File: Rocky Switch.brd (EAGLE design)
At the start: 81.1 x 50.2 mm, 40 parts, among them T1 BTA16, T2 BTA16, T3 BTA16, T4 BTA16

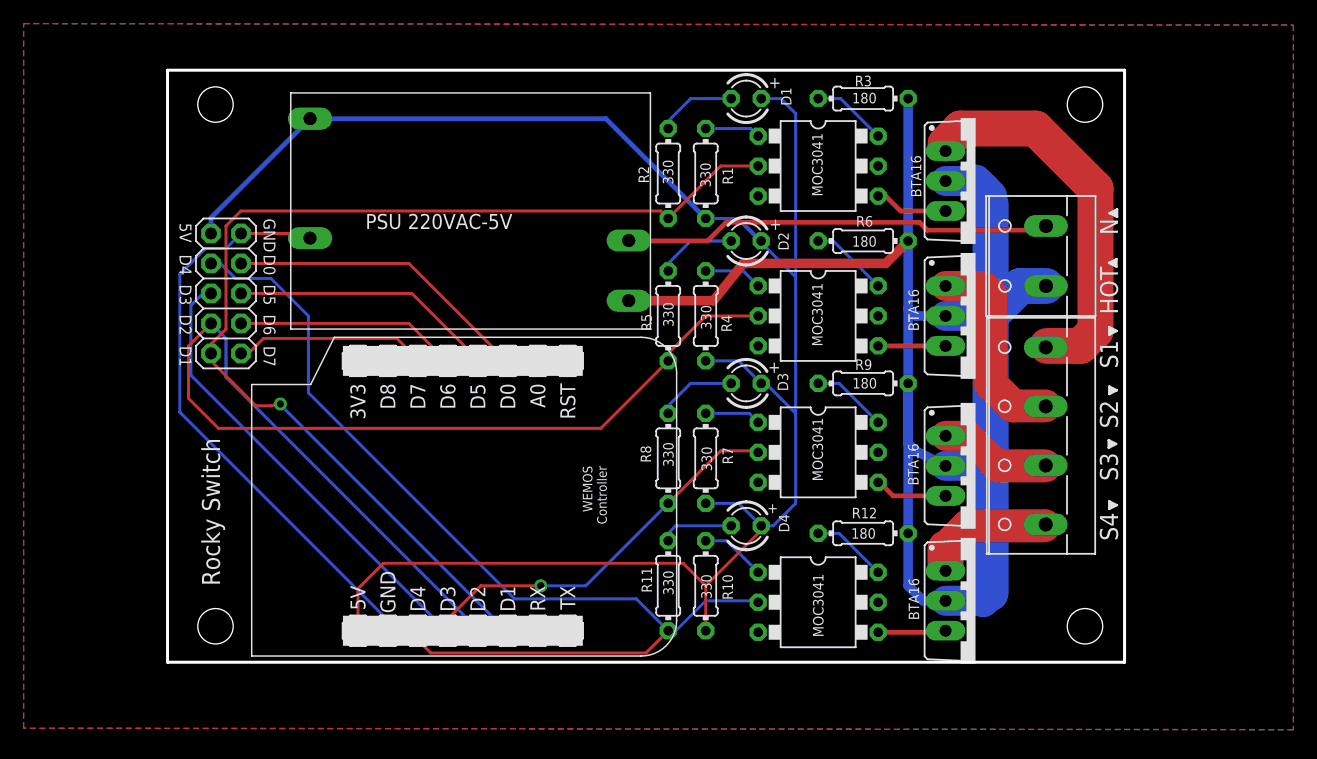
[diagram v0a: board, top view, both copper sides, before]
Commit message: Update board design to version 0.2
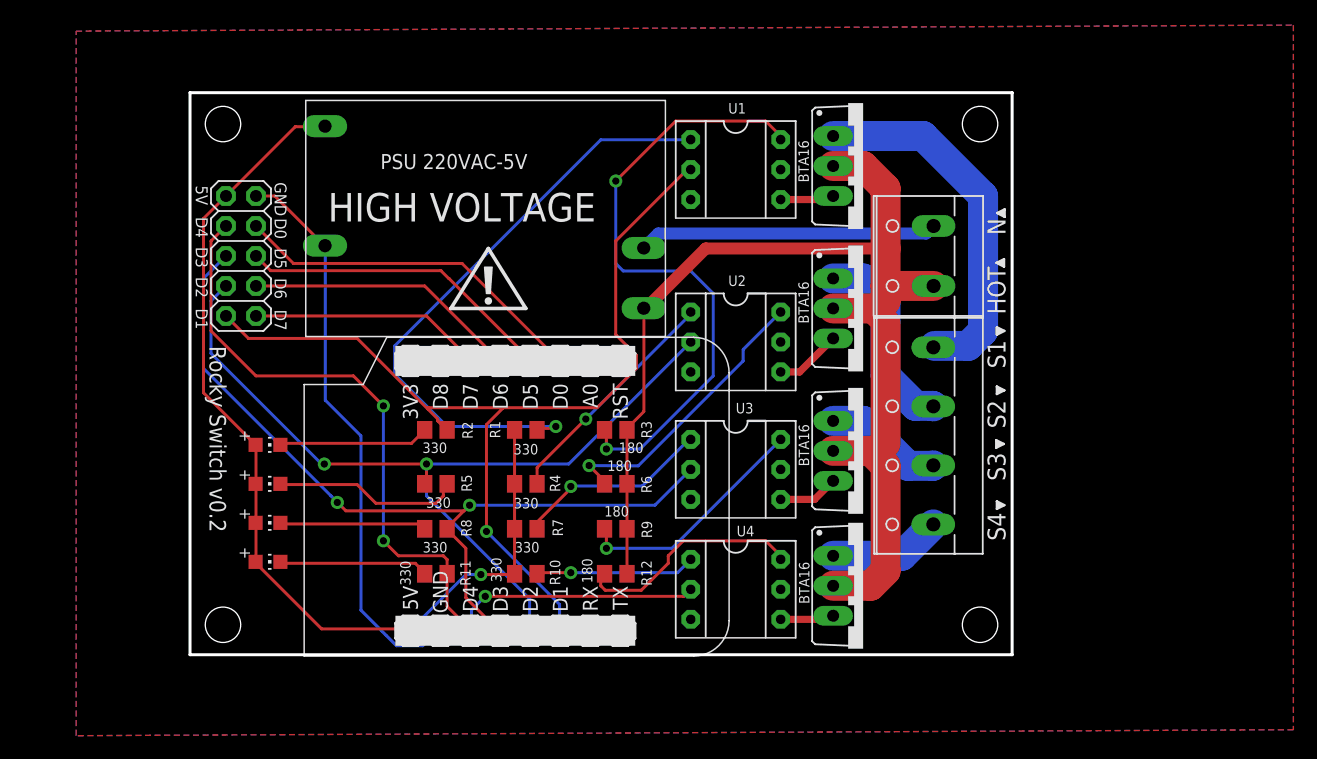
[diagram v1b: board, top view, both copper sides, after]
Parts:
- removed OK1, OK2, OK3, OK4: MOC3041, optocoupler:DIL06B
- added U1, U2, U3, U4: MOC3041, SparkFun-DiscreteSemi:DIL06
- D1: value (none) -> Relay1; device led:LED3MM -> adafruit:CHIP-LED0805
- D2: value (none) -> Relay2; device led:LED3MM -> adafruit:CHIP-LED0805
- D3: value (none) -> Relay3; device led:LED3MM -> adafruit:CHIP-LED0805
- D4: value (none) -> Relay4; device led:LED3MM -> adafruit:CHIP-LED0805
- R1, R10, R11, R12, R2, R3, R4, R5, R6, R7, R8, R9: device rcl:0204/7 -> rcl:R0805
- moved D1 50.0 mm to (9.27, 22.1), turned to 270 degrees
- moved D2 45.4 mm to (9.27, 18.8), turned to 270 degrees
- moved D3 42.2 mm to (9.27, 15.5), turned to 270 degrees
- moved D4 40.6 mm to (9.27, 12.2), turned to 270 degrees
- moved R3 35.0 mm to (38.7, 23.4)
- moved R6 29.4 mm to (38.7, 18.8)
- moved R2 29.3 mm to (23.5, 23.4), turned to 0 degrees
- moved R1 26.5 mm to (31.1, 23.4), turned to 0 degrees
- moved R9 24.3 mm to (38.7, 15.0)
- moved R5 24.3 mm to (23.5, 18.8), turned to 180 degrees
- moved U$17 21.3 mm to (27.9, 35.6), flipped to the top
- moved R12 21.2 mm to (38.7, 11.2)
- moved R4 20.8 mm to (31.1, 18.8), turned to 0 degrees
- moved R8 20.6 mm to (23.5, 15.0), turned to 0 degrees
- moved R11 19.7 mm to (23.5, 11.2), turned to 0 degrees
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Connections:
- net D1: now also U1.2; no longer OK1.2
- net D2: now also U2.2; no longer OK2.2
- net D3: now also U3.2; no longer OK3.2
- net D4: now also U4.2; no longer OK4.2
- net N$10: now also U1.1; no longer OK1.1
- net N$14: now also U1.6; no longer OK1.6
- net N$15: now also U2.4; no longer OK2.4
- net N$16: now also U2.1; no longer OK2.1
- net N$17: now also U2.6; no longer OK2.6
- net N$18: now also U3.4; no longer OK3.4
- net N$19: now also U3.1; no longer OK3.1
- net N$20: now also U3.6; no longer OK3.6
- net N$28: now also D1.C; no longer D1.K
- net N$29: now also D2.C; no longer D2.K
- net N$30: now also D3.C; no longer D3.K
- net N$32: now also U4.4; no longer OK4.4
- net N$33: now also U4.1; no longer OK4.1
- net N$34: now also U4.6; no longer OK4.6
- net N$38: now also D4.C; no longer D4.K
- net N$9: now also U1.4; no longer OK1.4
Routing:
- net 5V: track 163.9 -> 83.0 mm, vias 0 -> 1
- net AC_L: track 154.6 -> 104.9 mm
- net N$10: track 4.71 -> 52.0 mm, vias 0 -> 1
- net N$14: track 6.40 -> 53.6 mm, vias 0 -> 2
- net D2: track 96.0 -> 74.5 mm, vias 0 -> 2
- net N$17: track 6.66 -> 24.5 mm, vias 0 -> 1
- net D4: track 87.5 -> 71.9 mm, vias 0 -> 3
- net N$16: track 4.97 -> 20.0 mm, vias 0 -> 1
- net N$20: track 6.45 -> 20.4 mm, vias 0 -> 1
- net N$34: track 6.45 -> 19.7 mm
- net N$19: track 4.76 -> 16.8 mm, vias 0 -> 1
- net AC_N: track 36.4 -> 25.3 mm
- net D1: track 94.5 -> 84.5 mm
- net N$29: track 6.76 -> 16.0 mm
- net N$33: track 5.55 -> 13.6 mm, vias 0 -> 1
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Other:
- board size 81.1 x 50.2 mm -> 69.6 x 47.6 mm
- board text added: "Rocky Switch v0.2"
- board text removed: "+"
- board text removed: "Rocky Switch"
